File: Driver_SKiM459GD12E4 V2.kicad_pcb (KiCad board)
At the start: 4 copper layers, 169.2 x 116 mm, 340 parts, among them J1 2-338069-0, J13 EL1, J14 GL1, J15 NTC1_A, J16 NTC1_B, J17 GH1, J18 OUT1, J19 CH1, J20 EL2, J21 GL2, J22 NTC2_A, J23 NTC2_B, J24 GH2, J25 OUT2, J26 CH2, J27 EL3, J28 GL3, J29 NTC3_A, J30 NTC3_B, J31 GH3, J32 OUT3, J33 CH3, Q1 MJD44H11T4G, Q10 MJD45H11T4G, Q11 MJD44H11T4G, Q12 MJD45H11T4G, Q2 MJD45H11T4G, Q3 MJD44H11T4G, Q4 MJD45H11T4G, Q5 MJD44H11T4G, Q6 MJD45H11T4G, Q7 MJD44H11T4G, Q8 MJD45H11T4G, Q9 MJD44H11T4G, U1 LM2904, U2 R-785.0-1.0, U3 LM397, U4 HCPL-0611

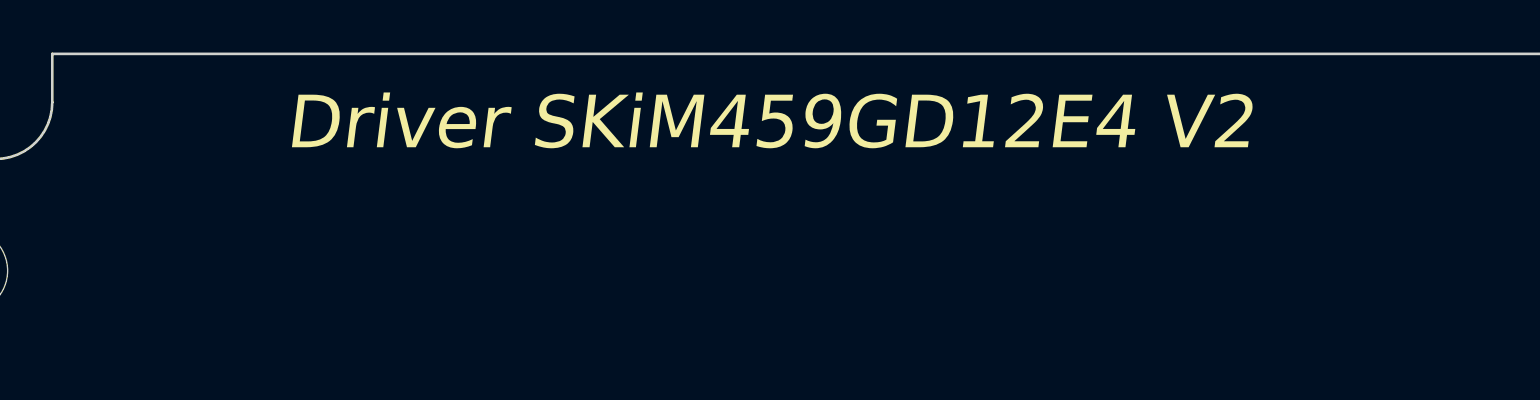
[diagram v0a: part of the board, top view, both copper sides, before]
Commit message: Нашёл ошибки
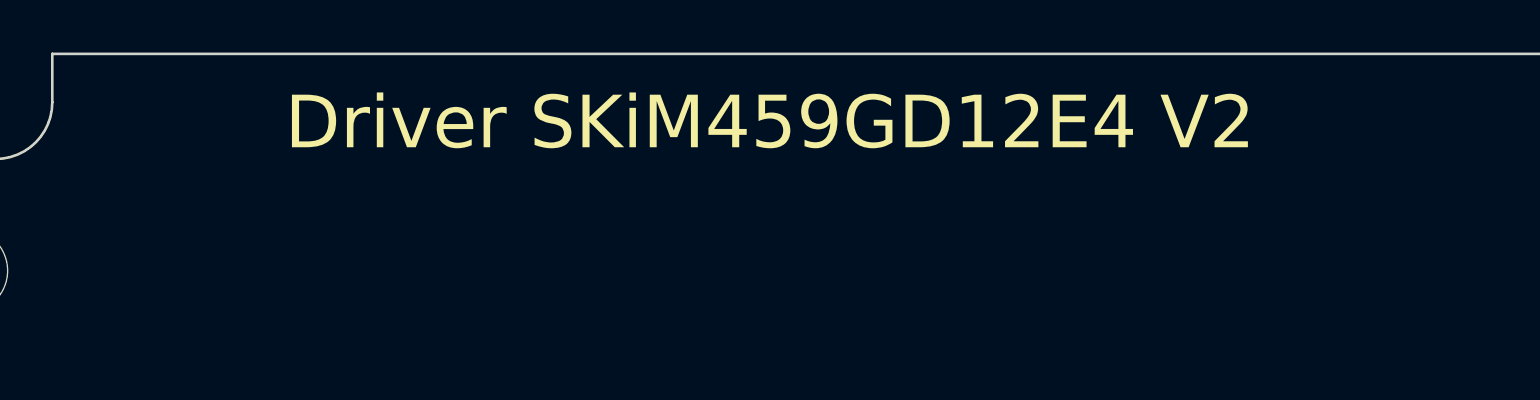
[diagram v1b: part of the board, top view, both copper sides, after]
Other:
- board text added: "1. Инвертировать ШИМ"
- board text added: "2. Исправить отверстия под крепления"
- board text added: "3. Инвертировать логику PTC"
- board text added: "4. Заменить R141 на 1,5кОм"
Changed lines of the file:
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@@
     (fp_line (start -0.227064 -0.735) (end 0.227064 -0.735) (layer "B.SilkS") (width 0.12))
     (fp_line (start -0.227064 0.735) (end 0.227064 0.735) (layer "B.SilkS") (width 0.12))
-    (fp_line (start -1.85 0.95) (end 1.85 0.95) (layer "B.CrtYd") (width 0.05))
     (fp_line (start 1.85 -0.95) (end -1.85 -0.95) (layer "B.CrtYd") (width 0.05))
+    (fp_line (start -1.85 0.95) (end 1.85 0.95) (layer "B.CrtYd") (width 0.05))
     (fp_line (start 1.85 0.95) (end 1.85 -0.95) (layer "B.CrtYd") (width 0.05))
     (fp_line (start -1.85 -0.95) (end -1.85 0.95) (layer "B.CrtYd") (width 0.05))
-    (fp_line (start -1 0.625) (end 1 0.625) (layer "B.Fab") (width 0.1))
-    (fp_line (start 1 -0.625) (end -1 -0.625) (layer "B.Fab") (width 0.1))
     (fp_line (start -1 -0.625) (end -1 0.625) (layer "B.Fab") (width 0.1))
+    (fp_line (start -1 0.625) (end 1 0.625) (layer "B.Fab") (width 0.1))
     (fp_line (start 1 0.625) (end 1 -0.625) (layer "B.Fab") (width 0.1))
+    (fp_line (start 1 -0.625) (end -1 -0.625) (layer "B.Fab") (width 0.1))
     (pad "1" smd roundrect (at -1 0 270) (size 1.2 1.4) (layers "B.Cu" "B.Paste" "B.Mask") (roundrect_rratio 0.208333)
       (net 166 "Net-(R101-Pad2)") (pintype "passive"))
@@
   )
   (gr_text "Driver SKiM459GD12E4 V2" (at 93.472 37.592) (layer "F.SilkS")
-    (effects (font (size 2 2) (thickness 0.4) italic))
+    (effects (font (size 2 2) (thickness 0.4)))
+  )
+  (gr_text "3. Инвертировать логику PTC" (at 95.25 176.725) (layer "User.1")
+    (effects (font (size 3 3) (thickness 0.45)))
+  )
+  (gr_text "1. Инвертировать ШИМ" (at 87.63 164.5) (layer "User.1")
+    (effects (font (size 3 3) (thickness 0.45)))
+  )
+  (gr_text "2. Исправить отверстия под крепления " (at 107.95 170.6) (layer "User.1")
+    (effects (font (size 3 3) (thickness 0.45)))
+  )
+  (gr_text "4. Заменить R141 на 1,5кОм" (at 95.25 182.88) (layer "User.1")
+    (effects (font (size 3 3) (thickness 0.45)))
   )
   (segment (start 107.9285 120.142) (end 107.9285 117.8935) (width 0.5) (layer "F.Cu") (net 1))
@@
   (segment (start 200.406 81.216) (end 201.74 82.55) (width 1) (layer "F.Cu") (net 19))
   (via (at 201.74 82.55) (size 0.8) (drill 0.4) (layers "F.Cu" "B.Cu") (net 19))
-  (segment (start 202.502 81.788) (end 201.74 82.55) (width 1) (layer "B.Cu") (net 19))
   (segment (start 205.46 81.788) (end 202.502 81.788) (width 1) (layer "B.Cu") (net 19))
+  (segment (start 202.502 81.788) (end 201.74 82.55) (width 1) (layer "B.Cu") (net 19))
   (segment (start 206.912 87.722) (end 201.74 82.55) (width 1) (layer "B.Cu") (net 19))
   (segment (start 210.309 60.325) (end 206.912 63.722) (width 0.5) (layer "B.Cu") (net 20))
